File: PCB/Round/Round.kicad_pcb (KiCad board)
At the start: 2 copper layers, 70 x 70 mm, 59 parts, among them J3 Conn, SW1 ESE13V01D, U1 PN532, U2 QR, Y1 27.12MHz

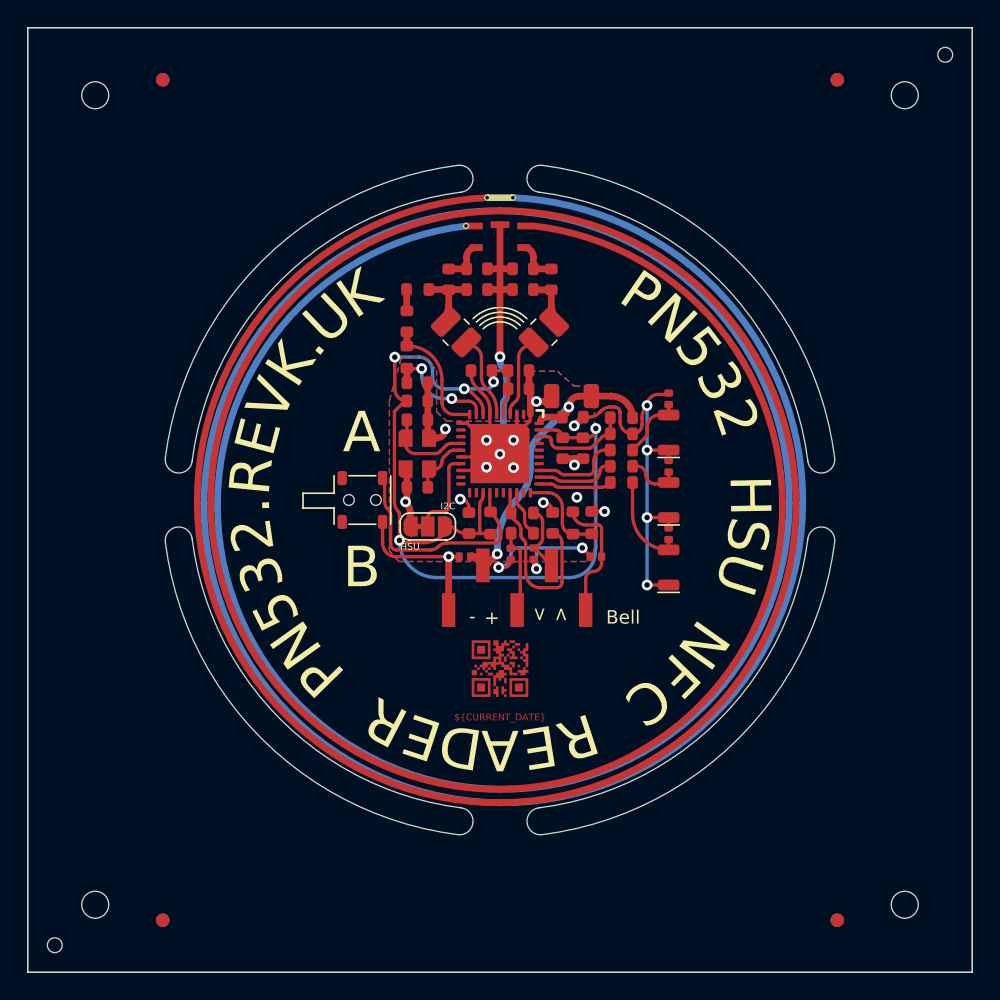
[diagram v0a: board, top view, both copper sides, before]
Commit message: PCB Update
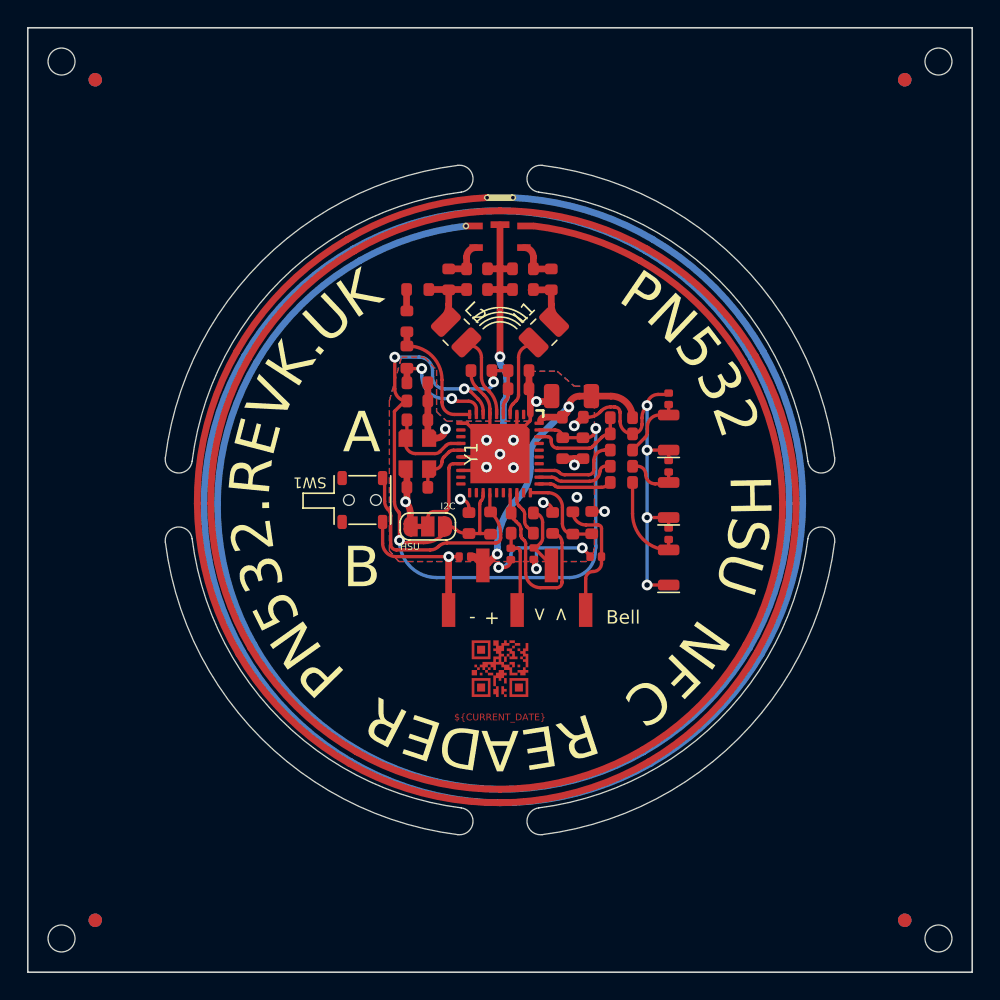
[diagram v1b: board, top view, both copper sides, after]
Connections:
- A1 pad 0: (no net) -> unconnected-(A1-LOOP-Pad0)_7
